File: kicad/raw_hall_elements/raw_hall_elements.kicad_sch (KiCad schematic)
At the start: 22 parts, among them IC1 AHE300G-PA4-B, IC2 AHE300G-PA4-B, U2 MCP6002-xMS

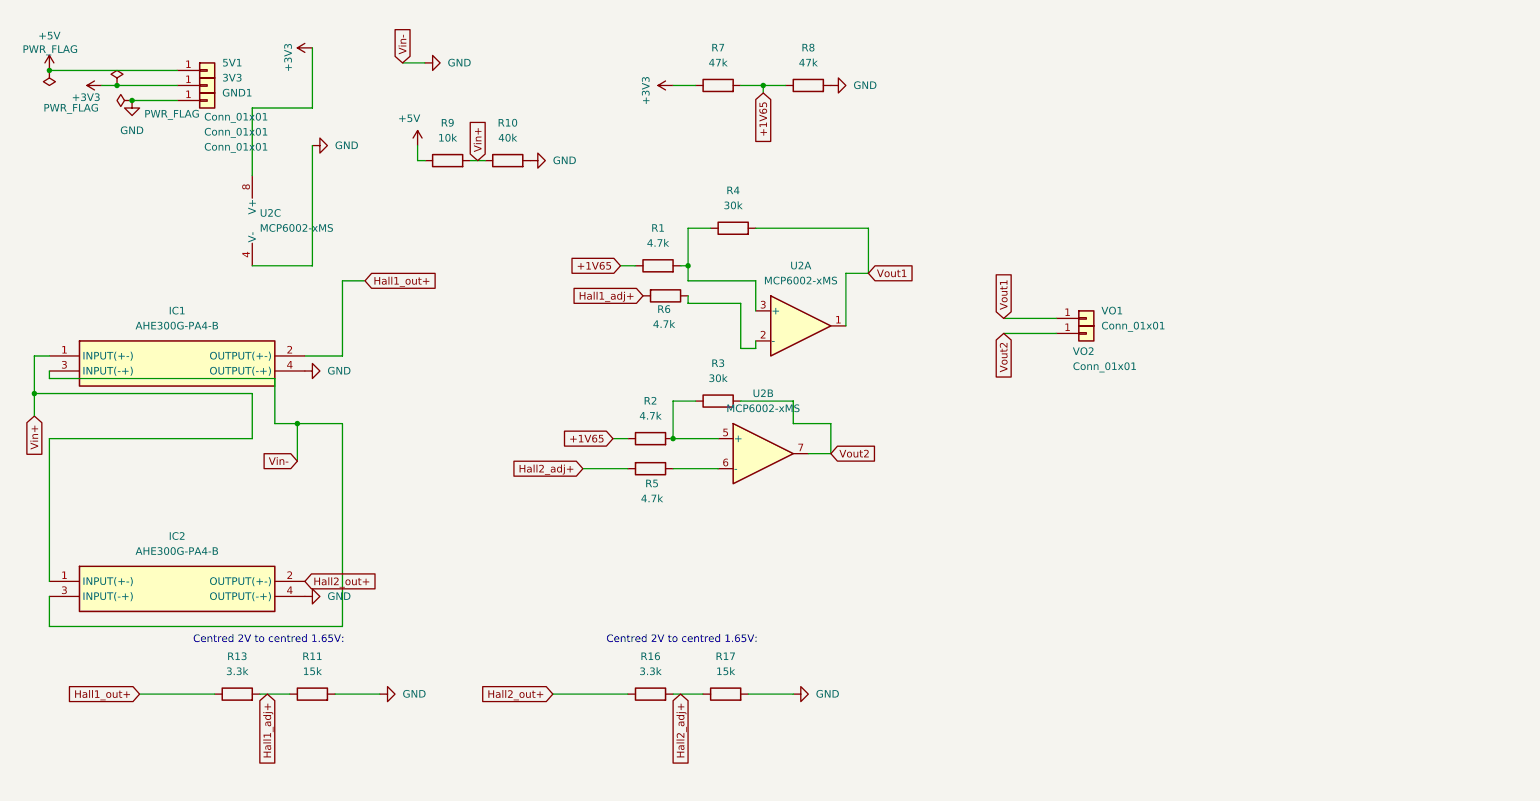
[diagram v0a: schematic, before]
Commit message: schematic clean up and layout finalise
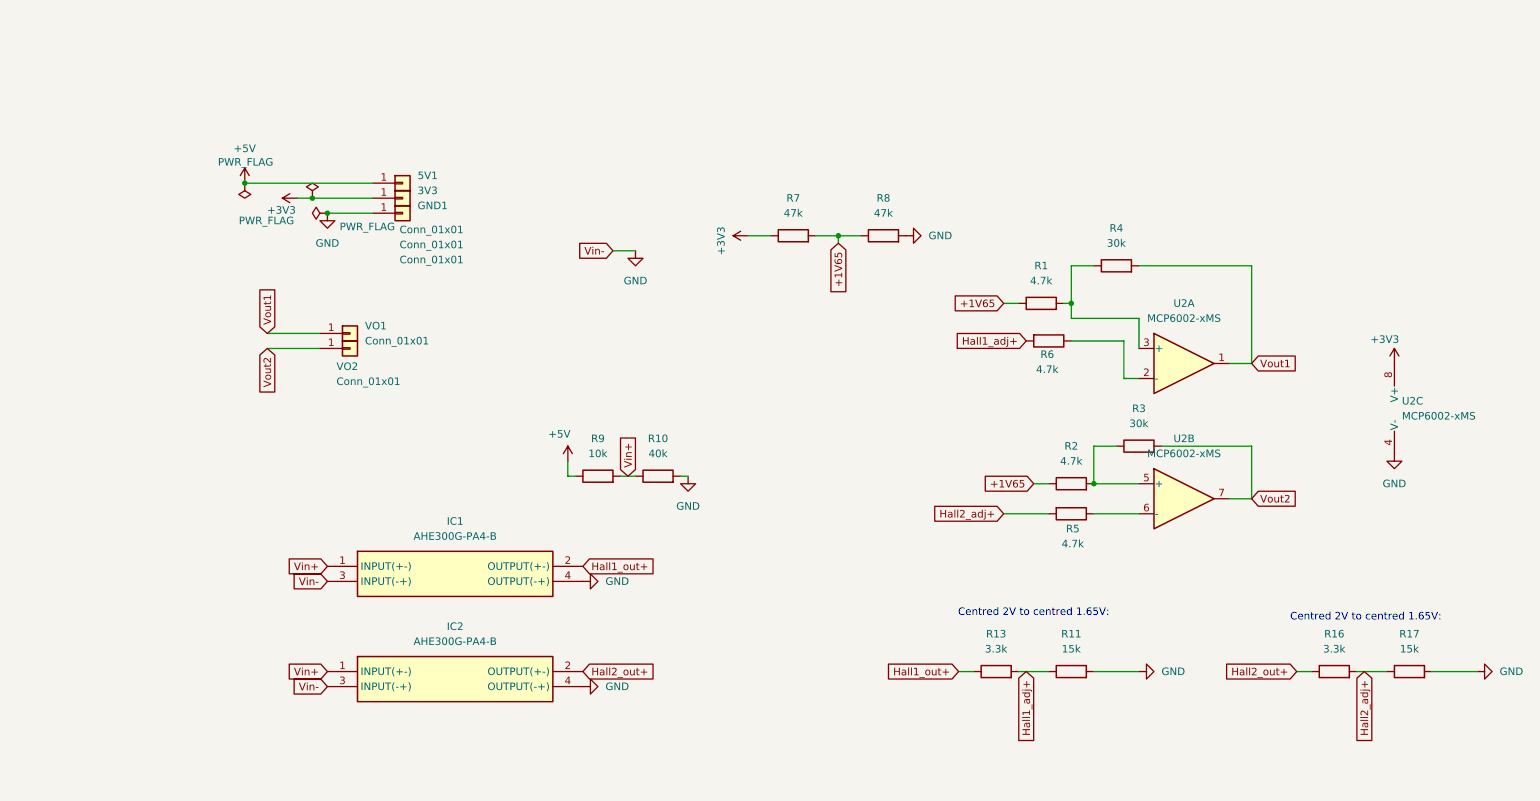
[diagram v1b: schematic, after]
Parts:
- 3V3, 5V1, GND1, VO1, VO2: footprint TestPoint:TestPoint_THTPad_1.0x1.0mm_Drill0.5mm -> TestPoint:TestPoint_THTPad_1.5x1.5mm_Drill0.7mm
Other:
- moved on the sheet: 3V3, 5V1, GND1, IC1, IC2, R1, R10, R11, R13, R16, R17, R2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
